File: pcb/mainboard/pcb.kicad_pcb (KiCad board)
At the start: 4 copper layers, 58 x 50 mm, 183 parts, among them J1 USB_B_Micro, J201 Conn_02x05_Odd_Even, J401 FH12-40S-0.5SH, J602 Molex_47272_DP, U200 XC6SLX16-FTG256, U202 W25X16JVP, U204 SY8008, U205 SY8008, U206 SY8008, U401 MAX17135, U502 MT41K64M16TW, U601 PTN3460, Y201 24MHz

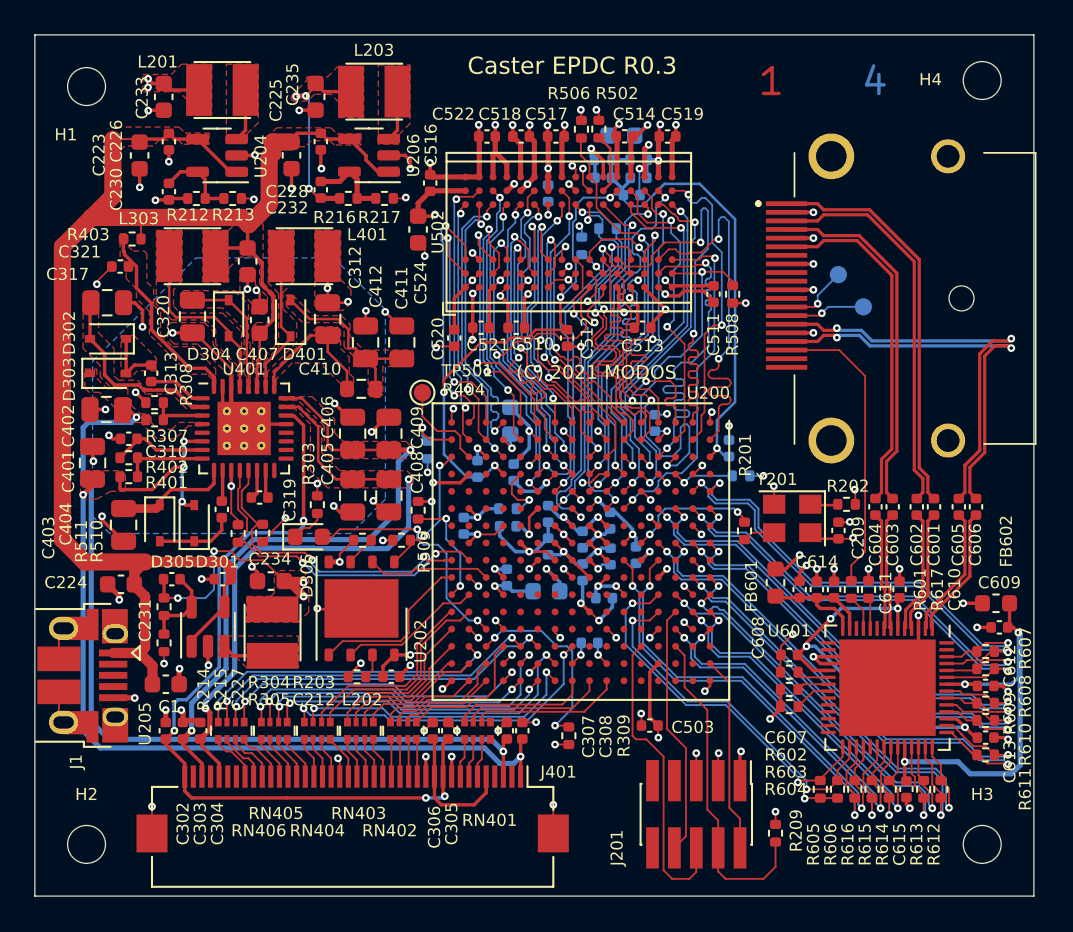
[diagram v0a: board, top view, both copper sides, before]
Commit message: pcb: r0p4
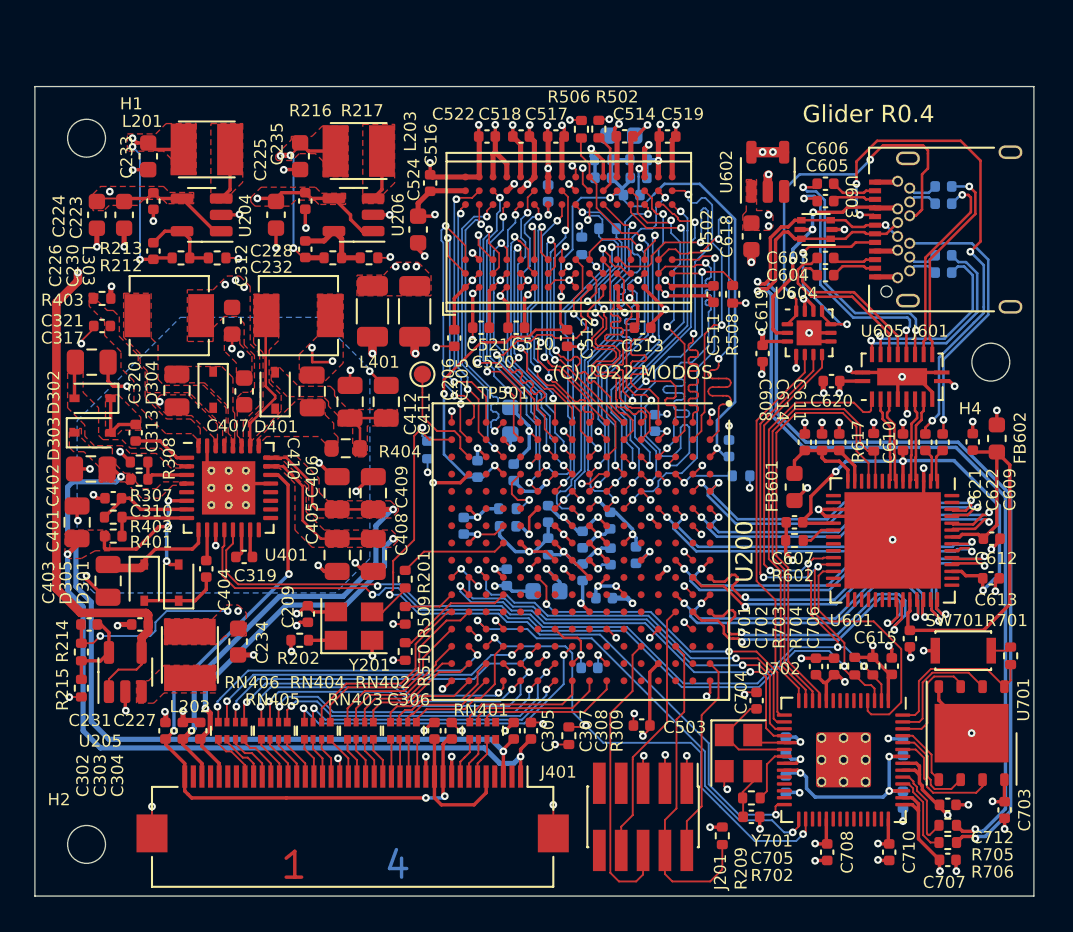
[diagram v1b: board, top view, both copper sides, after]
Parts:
- removed C1: 10uF, Capacitor_SMD:C_0603_1608Metric
- removed C212: 220nF, Capacitor_SMD:C_0402_1005Metric
- removed D306: LED, LED_SMD:LED_0603_1608Metric
- removed H3: MountingHole, MountingHole:MountingHole_2.2mm_M2_DIN965
- removed J1: USB_B_Micro, Connector_USB:USB_Micro-B_Amphenol_10103594-0001LF_Horizontal
- removed J602: Molex_47272_DP, footprints:472720024
- removed R203: 49.9K/1%, Resistor_SMD:R_0402_1005Metric
- removed R303: 1K, Resistor_SMD:R_0402_1005Metric
- removed R304, R305, R511, R603, R604: 4.7K, Resistor_SMD:R_0402_1005Metric
- removed R601: 0, Resistor_SMD:R_0402_1005Metric
- removed R605, R606: 10K, Resistor_SMD:R_0402_1005Metric
- removed R607, R608, R609, R610, R611, R612, R613, R614, R615, R616: 100, Resistor_SMD:R_0402_1005Metric
- removed TP601, TP602: TestPoint, TestPoint:TestPoint_Pad_D1.0mm
- removed U202: W25X16JVP, Package_SON:WSON-8-1EP_6x5mm_P1.27mm_EP3.4x4.3mm
- added C205: 100uF/6.3V, Capacitor_SMD:C_1206_3216Metric, F.Cu at (122.0, 66.0)
- added C206: 100uF/6.3V, Capacitor_SMD:C_1206_3216Metric, F.Cu at (119.6, 66.0)
- added C616: 100nF, Capacitor_SMD:C_0402_1005Metric, B.Cu at (152.8, 59.8)
- added C617: 100nF, Capacitor_SMD:C_0402_1005Metric, B.Cu at (152.8, 58.8)
- added C618: 10uF, Capacitor_SMD:C_0603_1608Metric, F.Cu at (141.6, 61.7)
- added C619: 100nF, Capacitor_SMD:C_0402_1005Metric, F.Cu at (142.2, 68.5)
- added C620: 100nF, Capacitor_SMD:C_0402_1005Metric, F.Cu at (146.2, 70.1)
- added C621: 100nF, Capacitor_SMD:C_0402_1005Metric, F.Cu at (151.7, 73.7)
- added C622: 100nF, Capacitor_SMD:C_0402_1005Metric, F.Cu at (152.7, 73.7)
- added C701: 1uF, Capacitor_SMD:C_0402_1005Metric, F.Cu at (145.3, 86.7)
- added C702: 100nF, Capacitor_SMD:C_0402_1005Metric, F.Cu at (146.4, 86.7)
- added C703: 100nF, Capacitor_SMD:C_0402_1005Metric, F.Cu at (156.3, 95.0)
- added C704: 18pF, Capacitor_SMD:C_0402_1005Metric, F.Cu at (141.9, 88.7)
- added C705: 18pF, Capacitor_SMD:C_0402_1005Metric, F.Cu at (141.6, 95.4)
- added C706: 100nF, Capacitor_SMD:C_0402_1005Metric, F.Cu at (149.7, 86.6)
- added C707: 100nF, Capacitor_SMD:C_0402_1005Metric, F.Cu at (153.0, 97.9)
- added C708: 100nF, Capacitor_SMD:C_0402_1005Metric, F.Cu at (146.0, 97.5)
- added C709: 100nF, Capacitor_SMD:C_0402_1005Metric, B.Cu at (143.6, 91.2)
- added C710: 100nF, Capacitor_SMD:C_0402_1005Metric, F.Cu at (149.6, 97.5)
- added C711: 100nF, Capacitor_SMD:C_0402_1005Metric, B.Cu at (150.4, 94.4)
- added C712: 100nF, Capacitor_SMD:C_0402_1005Metric, F.Cu at (153.0, 94.7)
- added C713: 100nF, Capacitor_SMD:C_0402_1005Metric, B.Cu at (143.6, 93.5)
- added C714: 1uF, Capacitor_SMD:C_0402_1005Metric, B.Cu at (150.4, 91.3)
- added J601: USB_C_Receptacle, Connector_USB:USB_C_Receptacle_Amphenol_12401548E4-2A, F.Cu at (153.8, 61.3)
- added R701: 1K, Resistor_SMD:R_0402_1005Metric, F.Cu at (156.7, 86.0)
- added R702: 1K, Resistor_SMD:R_0402_1005Metric, F.Cu at (141.6, 94.3)
- added R703: 4.7K, Resistor_SMD:R_0402_1005Metric, F.Cu at (147.6, 86.7)
- added R704: 4.7K, Resistor_SMD:R_0402_1005Metric, F.Cu at (148.7, 86.7)
- added R705: 27, Resistor_SMD:R_0402_1005Metric, F.Cu at (153.0, 95.9)
- added R706: 27, Resistor_SMD:R_0402_1005Metric, F.Cu at (153.0, 96.9)
- added SW701: EVQPUJ02K, Button_Switch_SMD:SW_SPST_CK_KXT3, F.Cu at (153.9, 85.8)
- added U602: TPS2001D, Package_TO_SOT_SMD:SOT-23-5, F.Cu at (142.6, 58.0)
- added U603: USBLC6-2P6, Package_TO_SOT_SMD:SOT-666, F.Cu at (145.3, 61.3)
- added U604: FUSB302BMPX, Package_DFN_QFN:WQFN-14-1EP_2.5x2.5mm_P0.5mm_EP1.45x1.45mm, F.Cu at (144.9, 67.3)
- added U605: CBTL02043A, Package_DFN_QFN:WQFN-20-1EP_2.5x4.5mm_P0.5mm_EP1x2.9mm, F.Cu at (150.3, 69.8)
- added U701: W25X16JVP, Package_SON:WSON-8-1EP_6x5mm_P1.27mm_EP3.4x4.3mm, F.Cu at (154.4, 90.5)
- added U702: RP2040, footprints:RP2040-QFN-56, F.Cu at (146.9, 92.1)
- added Y701: 12MHz, Oscillator:Oscillator_SMD_Abracon_ASE-4Pin_3.2x2.5mm, F.Cu at (140.8, 91.7)
- C601, C602: moved to B.Cu
- L303, L401: footprint footprints:L_1212 -> footprints:L_FXL0420
- R509, R510: value 4.7K -> 0
- U200: footprint Package_BGA:Xilinx_FTG256 -> footprints:Xilinx_FTG256
- moved R202 32.7 mm to (115.4, 85.1), turned to 0 degrees
- moved C209 31.2 mm to (115.8, 83.6), turned to 90 degrees
- moved Y201 26.2 mm to (118.5, 84.3), turned to 0 degrees
- moved C224 21.5 mm to (103.6, 60.5), turned to 90 degrees
- moved C606 20.7 mm to (145.9, 58.6), turned to 180 degrees
- moved R201 19.9 mm to (121.5, 81.6)
- moved C605 19.4 mm to (145.9, 59.6), turned to 180 degrees
- moved H4 16.4 mm to (155.5, 69.0)
- moved C603 15.0 mm to (145.9, 63.0), turned to 180 degrees
- moved C601 14.6 mm to (152.8, 62.8), turned to 0 degrees
- moved C604 13.8 mm to (145.9, 64.0), turned to 180 degrees
- moved C602 13.7 mm to (152.8, 63.8), turned to 0 degrees
- moved C609 10.9 mm to (154.4, 73.6), turned to 90 degrees
- moved R510 10.8 mm to (121.5, 85.8)
- moved FB602 9.57 mm to (155.8, 73.4), turned to -90 degrees
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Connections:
- C601 pad 1: /dp_in/D0P -> /dp_in/TX1N
- C601 pad 2: /dp_in/DP0P -> /dp_in/TX1NC
- C602 pad 1: /dp_in/D0N -> /dp_in/TX1P
- C602 pad 2: /dp_in/DP0N -> /dp_in/TX1PC
- C603 pad 1: /dp_in/D1P -> /dp_in/RX1N
- C603 pad 2: /dp_in/DP1P -> /dp_in/RX1NC
- C604 pad 1: /dp_in/D1N -> /dp_in/RX1P
- C604 pad 2: /dp_in/DP1N -> /dp_in/RX1PC
- C605 pad 1: /dp_in/AUXP -> /dp_in/TX2N
- C605 pad 2: /dp_in/DPAUXP -> /dp_in/TX2NC
- C606 pad 1: /dp_in/AUXN -> /dp_in/TX2P
- C606 pad 2: /dp_in/DPAUXN -> /dp_in/TX2PC
- R201 pad 1: /fpga/GCLK -> GCLK
- R510 pad 2: EPD_PWR_SDA -> Net-(U200-PadN11)
- R617 pad 1: +3V3 -> GND
- U200 pad A13: LVDS_EVEN_CKN -> unconnected-(U200-PadA13)
- U200 pad A8: LVDS_ODD_CKN -> unconnected-(U200-PadA8)
- U200 pad A9: unconnected-(U200-PadA9) -> LVDS_ODD_CKN
- U200 pad B8: LVDS_ODD_CKP -> unconnected-(U200-PadB8)
- U200 pad C13: LVDS_EVEN_CKP -> unconnected-(U200-PadC13)
- U200 pad C8: LVDS_ODD_DN -> unconnected-(U200-PadC8)
- U200 pad C9: unconnected-(U200-PadC9) -> LVDS_ODD_CKP
- U200 pad D11: DDC_SCL -> unconnected-(U200-PadD11)
- U200 pad D12: DDC_SDA -> unconnected-(U200-PadD12)
- U200 pad D8: LVDS_ODD_DP -> unconnected-(U200-PadD8)
- U200 pad D9: LVDS_EVEN_DN -> unconnected-(U200-PadD9)
- U200 pad E8: /fpga/GCLK -> unconnected-(U200-PadE8)
- U200 pad F9: LVDS_EVEN_DP -> unconnected-(U200-PadF9)
- U200 pad L10: unconnected-(U200-PadL10) -> FPGA_CS
- U200 pad N11: GND -> Net-(U200-PadN11)
- U200 pad N8: unconnected-(U200-PadN8) -> GCLK
- U200 pad P10: FPGA_FMISO -> FPGA_MOSI
- U200 pad P13: /fpga/FPGA_DONE -> FPGA_DONE
- U200 pad R11: FPGA_FCCLK -> FPGA_SCLK
- U200 pad R9: EPD_PWR_SCL -> unconnected-(U200-PadR9)
- U200 pad T10: FPGA_FMOSI -> FPGA_MISO
- U200 pad T3: FPGA_FCS -> unconnected-(U200-PadT3)
- U200 pad T9: EPD_PWR_SDA -> unconnected-(U200-PadT9)
- U401 pad 12: EPD_PWR_SCL -> I2C_SCL
- U401 pad 13: EPD_PWR_SDA -> I2C_SDA
- U601 pad 11: Net-(R601-Pad2) -> DP_HPD
- U601 pad 21: Net-(R603-Pad2) -> unconnected-(U601-Pad21)
- U601 pad 22: Net-(R604-Pad2) -> unconnected-(U601-Pad22)
- U601 pad 26: unconnected-(U601-Pad26) -> DP_VALID
- U601 pad 29: DDC_SCL -> unconnected-(U601-Pad29)
- U601 pad 30: DDC_SDA -> unconnected-(U601-Pad30)
- U601 pad 31: LVDS_EVEN_DP -> unconnected-(U601-Pad31)
- U601 pad 32: LVDS_EVEN_DN -> unconnected-(U601-Pad32)
- U601 pad 34: LVDS_EVEN_CKP -> unconnected-(U601-Pad34)
- U601 pad 35: LVDS_EVEN_CKN -> unconnected-(U601-Pad35)
- U601 pad 43: LVDS_ODD_DP -> unconnected-(U601-Pad43)
- U601 pad 44: LVDS_ODD_DN -> unconnected-(U601-Pad44)
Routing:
- net I2C_SCL: track 0.00 -> 71.4 mm, vias 0 -> 4
- net I2C_SDA: track 0.00 -> 69.8 mm, vias 0 -> 5
- net USB_DN: track 0.00 -> 57.8 mm, vias 0 -> 3
- net USB_DP: track 0.00 -> 56.8 mm, vias 0 -> 2
- net +5V: track 98.9 -> 47.7 mm, vias 0 -> 12
- net FPGA_PROG: track 3.08 -> 43.7 mm, vias 1 -> 3
- net +3V3: track 62.2 -> 95.4 mm, vias 40 -> 48
- net LVDS_ODD_DP: track 30.4 -> 0.00 mm, vias 2 -> 0
- net /dp_in/SBU1: track 0.00 -> 30.1 mm, vias 0 -> 4
- net LVDS_ODD_DN: track 30.0 -> 0.00 mm, vias 2 -> 0
- net LVDS_EVEN_DP: track 27.0 -> 0.00 mm, vias 2 -> 0
- net LVDS_EVEN_DN: track 26.3 -> 0.00 mm, vias 2 -> 0
- net FPGA_DONE: track 0.00 -> 26.2 mm, vias 0 -> 2
- net FPGA_MISO: track 0.00 -> 25.6 mm, vias 0 -> 2
- net DP_HPD: track 0.00 -> 25.5 mm
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- added copper zone on In1.Cu, net +5V
- added copper zone on In1.Cu, net /dp_in/VBUS
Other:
- board size 58 x 50 mm -> 58 x 47 mm
- board text added: "(C) 2022 MODOS"
- board text added: "Glider R0.4"
- board text removed: "(C) 2021 MODOS"
- board text removed: "Caster EPDC R0.3"

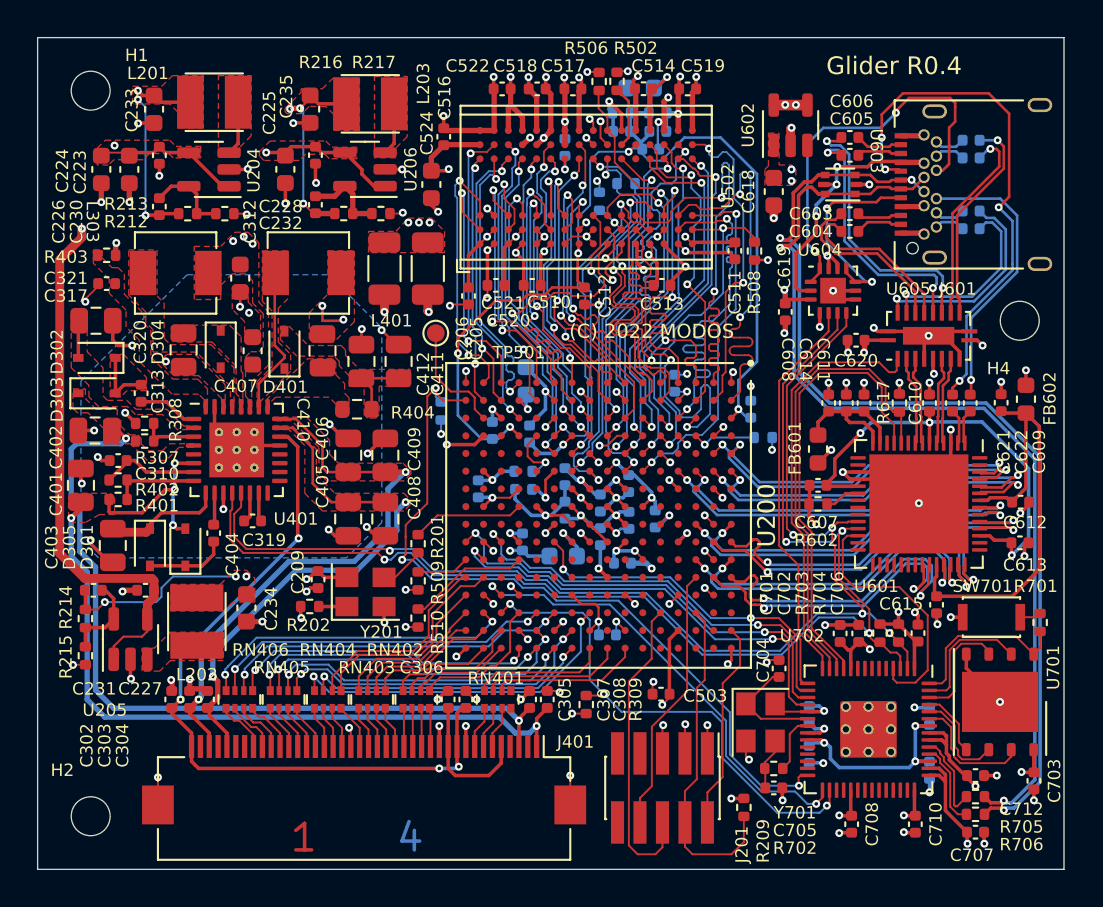
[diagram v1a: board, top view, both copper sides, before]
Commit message: pcb: r0p5
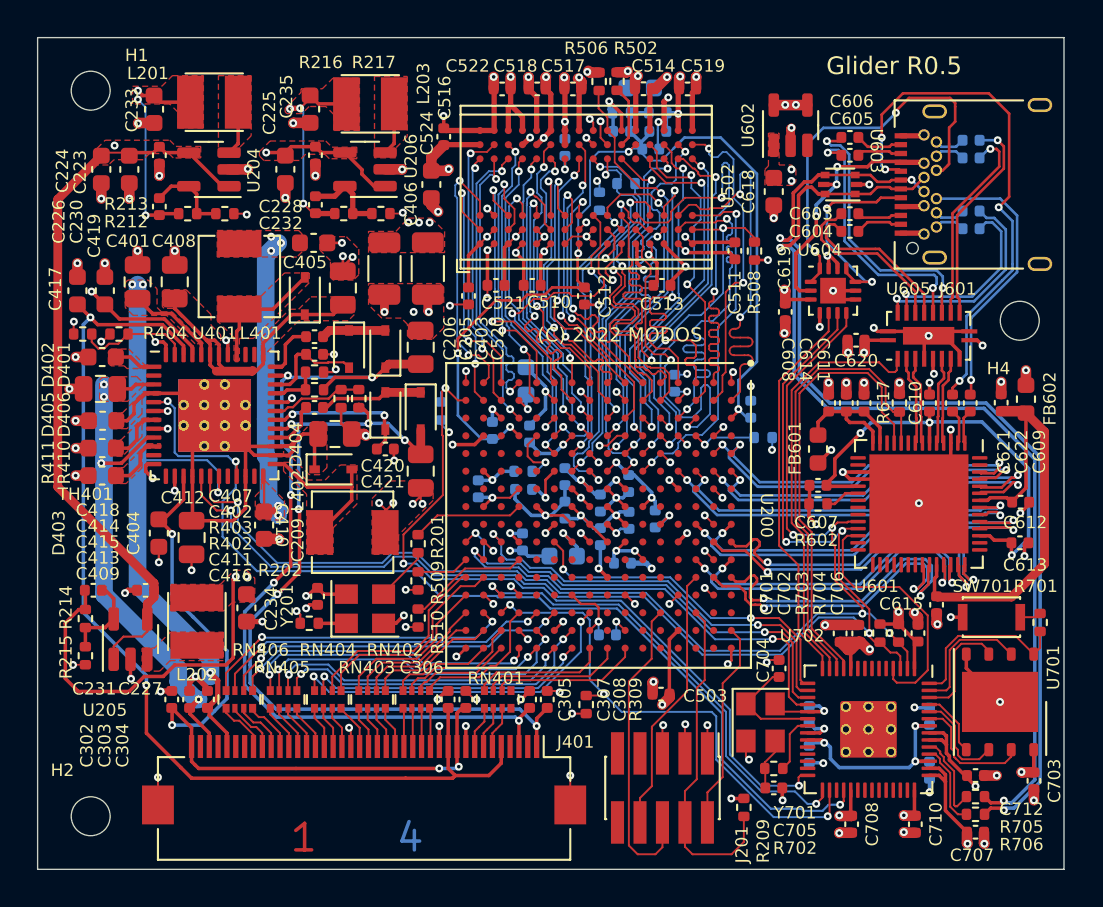
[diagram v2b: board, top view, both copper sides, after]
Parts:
- removed C310, C313: 100nF, Capacitor_SMD:C_0402_1005Metric
- removed C312: 10uF, Capacitor_SMD:C_0603_1608Metric
- removed C317: 1uF/25V, Capacitor_SMD:C_0805_2012Metric
- removed C319: 2.2nF, Capacitor_SMD:C_0402_1005Metric
- removed C320: 4.7uF/25V, Capacitor_SMD:C_0805_2012Metric
- removed C321: 1uF, Capacitor_SMD:C_0402_1005Metric
- removed D301, D302, D303, D304, D305: B0530WS, Diode_SMD:D_SOD-323
- removed L303: 4.7uH, footprints:L_FXL0420
- removed R307: 562K/1%, Resistor_SMD:R_0402_1005Metric
- removed R308: 27K/1%, Resistor_SMD:R_0402_1005Metric
- removed R401: 806K/1%, Resistor_SMD:R_0402_1005Metric
- removed TP501: TestPoint, TestPoint:TestPoint_Pad_D1.0mm
- added C413: 4.7uF, Capacitor_SMD:C_0603_1608Metric, F.Cu at (103.7, 76.2)
- added C414: 4.7uF, Capacitor_SMD:C_0603_1608Metric, F.Cu at (103.7, 71.0)
- added C415: 4.7uF, Capacitor_SMD:C_0603_1608Metric, F.Cu at (103.7, 74.7)
- added C416: 4.7uF/25V, Capacitor_SMD:C_0805_2012Metric, F.Cu at (116.8, 75.4)
- added C417: 4.7uF, Capacitor_SMD:C_0603_1608Metric, F.Cu at (102.2, 67.3)
- added C418: 4.7uF/25V, Capacitor_SMD:C_0805_2012Metric, F.Cu at (103.5, 72.8)
- added C419: 4.7uF, Capacitor_SMD:C_0603_1608Metric, F.Cu at (103.8, 67.3)
- added C420: 100nF, Capacitor_SMD:C_0402_1005Metric, F.Cu at (119.7, 76.2)
- added C421: 4.7uF/25V, Capacitor_SMD:C_0805_2012Metric, F.Cu at (121.7, 77.5)
- added D402: B0530WS, Diode_SMD:D_SOD-323, F.Cu at (117.6, 70.6)
- added D403: B0530WS, Diode_SMD:D_SOD-323, F.Cu at (115.1, 67.6)
- added D404: B0530WS, Diode_SMD:D_SOD-323, F.Cu at (116.7, 77.4)
- added D405: B0530WS, Diode_SMD:D_SOD-323, F.Cu at (119.7, 74.1)
- added D406: B0530WS, Diode_SMD:D_SOD-323, F.Cu at (121.7, 74.1)
- added L402: FXL0420-4R7-M, footprints:L_FXL0420, F.Cu at (117.8, 81.0)
- added R410: 510K/1%, Resistor_SMD:R_0402_1005Metric, F.Cu at (118.2, 73.4)
- added R411: 24K/1%, Resistor_SMD:R_0402_1005Metric, F.Cu at (117.2, 73.4)
- added TH401: 10K, Resistor_SMD:R_0402_1005Metric, F.Cu at (102.5, 69.8)
- C401, C403: value 1uF/25V -> 4.7uF/25V
- C402: value 1uF/25V -> 100nF; footprint Capacitor_SMD:C_0805_2012Metric -> Capacitor_SMD:C_0402_1005Metric
- C404: value 100nF -> 4.7uF; footprint Capacitor_SMD:C_0402_1005Metric -> Capacitor_SMD:C_0603_1608Metric
- C405, C410: value 4.7uF/25V -> 10uF; footprint Capacitor_SMD:C_0805_2012Metric -> Capacitor_SMD:C_0603_1608Metric
- C407: value 10uF -> 10nF; footprint Capacitor_SMD:C_0603_1608Metric -> Capacitor_SMD:C_0402_1005Metric
- C409: value 4.7uF/25V -> 4.7uF; footprint Capacitor_SMD:C_0805_2012Metric -> Capacitor_SMD:C_0603_1608Metric
- C411: value 4.7uF/25V -> 10nF; footprint Capacitor_SMD:C_0805_2012Metric -> Capacitor_SMD:C_0402_1005Metric
- L401: value 4.7uH -> FXL0420-2R2-M
- R201: value 22R -> 27
- R402: value 49.9K/1% -> 470K/1%
- R403: value 10R -> 18K/1%
- R404: value 0.5R -> 43K; footprint Resistor_SMD:R_0603_1608Metric -> Resistor_SMD:R_0402_1005Metric
- U401: value MAX17135 -> TPS65185; footprint Package_DFN_QFN:QFN-32-1EP_5x5mm_P0.5mm_EP3.1x3.1mm_ThermalVias -> footprints:QFN-48-1EP_7x7mm_P0.5mm_EP4.1x4.1mm_ThermalVias
- U701: value W25X16JVP -> W25Q32JV
- Y201: value 24MHz -> 33MHz
- moved C403 20.7 mm to (121.7, 70.5), turned to -90 degrees
- moved C408 17.9 mm to (107.8, 66.8), turned to -90 degrees
- moved C409 16.0 mm to (103.7, 77.8), turned to 0 degrees
- moved C405 15.7 mm to (115.6, 64.6), turned to 180 degrees
- moved R404 14.1 mm to (104.6, 69.8), turned to 0 degrees
- moved C412 13.8 mm to (108.7, 81.2)
- moved R403 13.5 mm to (115.7, 71.9)
- moved C402 13.1 mm to (115.7, 70.9), turned to 180 degrees
- moved R402 12.2 mm to (115.7, 72.9), turned to 180 degrees
- moved C401 11.9 mm to (105.7, 66.8)
- moved C410 10.4 mm to (112.8, 80.5)
- moved C406 9.45 mm to (117.2, 67.2)
- moved D401 5.70 mm to (119.7, 70.6)
- moved C411 5.42 mm to (115.7, 73.9), turned to 0 degrees
- moved L401 3.91 mm to (111.4, 66.5), turned to -90 degrees
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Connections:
- C401 pad 1: GNDPWR -> GND
- C401 pad 2: VGL -> VPOS
- C402 pad 1: GNDPWR -> GND
- C402 pad 2: VGH -> Net-(D402-Pad2)
- C403 pad 1: GNDPWR -> GND
- C403 pad 2: Net-(C403-Pad2) -> VGH
- C404 pad 1: Net-(C404-Pad1) -> GND
- C404 pad 2: Net-(C404-Pad2) -> VCOM
- C405 pad 1: GNDPWR -> GND
- C405 pad 2: VPOS -> +5V
- C406 pad 1: GNDPWR -> GND
- C406 pad 2: VNEG -> Net-(C406-Pad2)
- C407 pad 1: GNDPWR -> Net-(C407-Pad1)
- C407 pad 2: +5V -> Net-(C407-Pad2)
- C408 pad 1: GNDPWR -> GND
- C408 pad 2: VPOS -> Net-(C406-Pad2)
- C409 pad 1: GNDPWR -> GND
- C409 pad 2: VNEG -> IPSOUT
- C410 pad 1: GNDPWR -> +5V
- C410 pad 2: Net-(C410-Pad2) -> GND
- C411 pad 1: GNDPWR -> Net-(C411-Pad1)
- C412 pad 1: GNDPWR -> Net-(C415-Pad1)
- C412 pad 2: Net-(C411-Pad2) -> GND
- D401 pad 1: Net-(D401-Pad1) -> VGH
- D401 pad 2: Net-(C411-Pad2) -> Net-(C407-Pad1)
- L401 pad 1: Net-(D401-Pad1) -> +5V
- L401 pad 2: GNDPWR -> Net-(L401-Pad2)
- R402 pad 1: Net-(C310-Pad2) -> VGH
- R402 pad 2: Net-(R401-Pad2) -> Net-(R402-Pad2)
- R403 pad 1: Net-(C321-Pad2) -> Net-(R402-Pad2)
- R403 pad 2: +5V -> GND
- R404 pad 1: Net-(C411-Pad2) -> GND
- R404 pad 2: Net-(C410-Pad2) -> Net-(R404-Pad2)
- U401 pad 10: Net-(C404-Pad2) -> IPSOUT
- U401 pad 11: +3V3 -> unconnected-(U401-Pad11)
- U401 pad 12: I2C_SCL -> +3V3
- U401 pad 13: I2C_SDA -> unconnected-(U401-Pad13)
- U401 pad 14: Net-(C319-Pad2) -> GND
- U401 pad 15: Net-(C319-Pad1) -> VCOM
- U401 pad 16: unconnected-(U401-Pad16) -> Net-(C415-Pad1)
- U401 pad 17: unconnected-(U401-Pad17) -> I2C_SCL
- U401 pad 18: unconnected-(U401-Pad18) -> I2C_SDA
- U401 pad 19: unconnected-(U401-Pad19) -> VPOS
- U401 pad 2: Net-(C317-Pad1) -> unconnected-(U401-Pad2)
- U401 pad 21: GND -> EPD_PWR_EN
- U401 pad 22: VCOM -> Net-(C415-Pad1)
- U401 pad 23: VPOS -> /eink/EPD_PWROK
- U401 pad 24: VNEG -> +5V
- U401 pad 25: Net-(C410-Pad2) -> Net-(D404-Pad2)
- U401 pad 26: Net-(D401-Pad1) -> Net-(C415-Pad1)
- U401 pad 27: +5V -> Net-(C415-Pad1)
- U401 pad 28: Net-(C320-Pad2) -> Net-(C411-Pad1)
- U401 pad 29: Net-(D304-Pad2) -> VGL
- U401 pad 3: Net-(R307-Pad2) -> VNEG
- U401 pad 30: GNDPWR -> Net-(C420-Pad1)
- U401 pad 31: GND -> Net-(R410-Pad2)
- U401 pad 32: Net-(C321-Pad2) -> GND
- U401 pad 33: GND -> Net-(R402-Pad2)
- U401 pad 4: VGH -> Net-(C415-Pad1)
- U401 pad 5: unconnected-(U401-Pad5) -> EPD_PWR_EN
- U401 pad 6: VGL -> GND
- U401 pad 7: Net-(C310-Pad2) -> Net-(C413-Pad1)
- U401 pad 8: Net-(R401-Pad2) -> GND
- U401 pad 9: Net-(C403-Pad2) -> VNEG
- U604 pad 12: +3V3 -> GND
- U604 pad 13: +3V3 -> GND
- U702 pad 32: /mcu/GPIO21 -> EPD_PWR_EN
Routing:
- net EPD_PWR_EN: track 0.00 -> 56.9 mm, vias 0 -> 3
- net +3V3_LCD: track 7.86 -> 59.0 mm, vias 0 -> 2
- net Net-(C415-Pad1): track 0.00 -> 34.4 mm
- net GND: track 206.9 -> 236.0 mm, vias 133 -> 163
- net +5V: track 47.7 -> 69.3 mm
- net Net-(C406-Pad2): track 0.00 -> 19.1 mm
- net GNDPWR: track 16.4 -> 0.00 mm, vias 15 -> 0
- net VPOS: track 30.0 -> 41.1 mm, vias 2 -> 4
- net +1V1: track 27.0 -> 37.3 mm, vias 8 -> 7
- net +3V3: track 95.4 -> 104.7 mm
- net Net-(D404-Pad2): track 0.00 -> 9.15 mm
- net Net-(C420-Pad1): track 0.00 -> 8.57 mm, vias 0 -> 2
- net Net-(D401-Pad1): track 8.39 -> 0.00 mm
- net Net-(L401-Pad2): track 0.00 -> 7.07 mm
- net Net-(C403-Pad2): track 6.76 -> 0.00 mm
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- added copper zone on F.Cu, net GND
- added copper zone on F.Cu, net IPSOUT
- added copper zone on F.Cu, net Net-(C406-Pad2)
- added copper zone on F.Cu, net Net-(C413-Pad1)
- added copper zone on F.Cu, net Net-(C414-Pad1)
- added copper zone on F.Cu, net Net-(C415-Pad1)
- added copper zone on F.Cu, net Net-(D404-Pad2)
- added copper zone on F.Cu, net Net-(L401-Pad2)
- removed copper zone on B.Cu, net GNDPWR
- removed copper zone on F.Cu, net GNDPWR
- removed copper zone on F.Cu, net Net-(C313-Pad1)
- removed copper zone on F.Cu, net Net-(C317-Pad1)
- removed copper zone on F.Cu, net Net-(C320-Pad2)
- removed copper zone on F.Cu, net Net-(C321-Pad2)
- removed copper zone on F.Cu, net Net-(C410-Pad2)
- removed copper zone on F.Cu, net Net-(C411-Pad2)
- removed copper zone on F.Cu, net Net-(D304-Pad2)
- removed copper zone on F.Cu, net Net-(D401-Pad1)
- removed copper zone on F.Cu, net VGH
- removed copper zone on F.Cu, net VGL
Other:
- board text added: "Glider R0.5"
- board text removed: "Glider R0.4"
